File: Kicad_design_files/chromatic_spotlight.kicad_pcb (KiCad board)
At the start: 2 copper layers, 29.7 x 29.7 mm, 35 parts, among them CON1 POWER_CONN, P1 CONN_6, Q1 MOSFET_N, Q2 MOSFET_N, SW1 SLIDE 1PDT, U1 LT3474, U2 LT3474

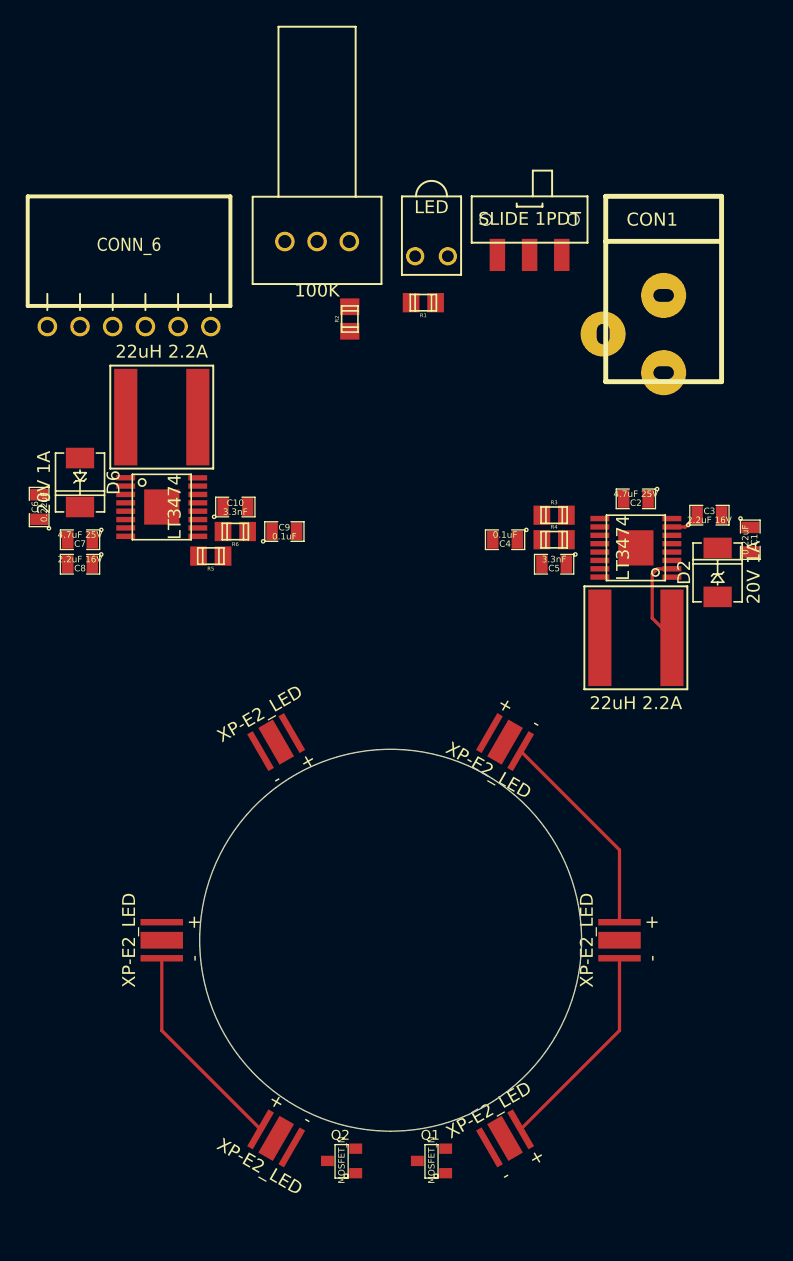
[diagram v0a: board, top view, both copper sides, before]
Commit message: almost done with layout
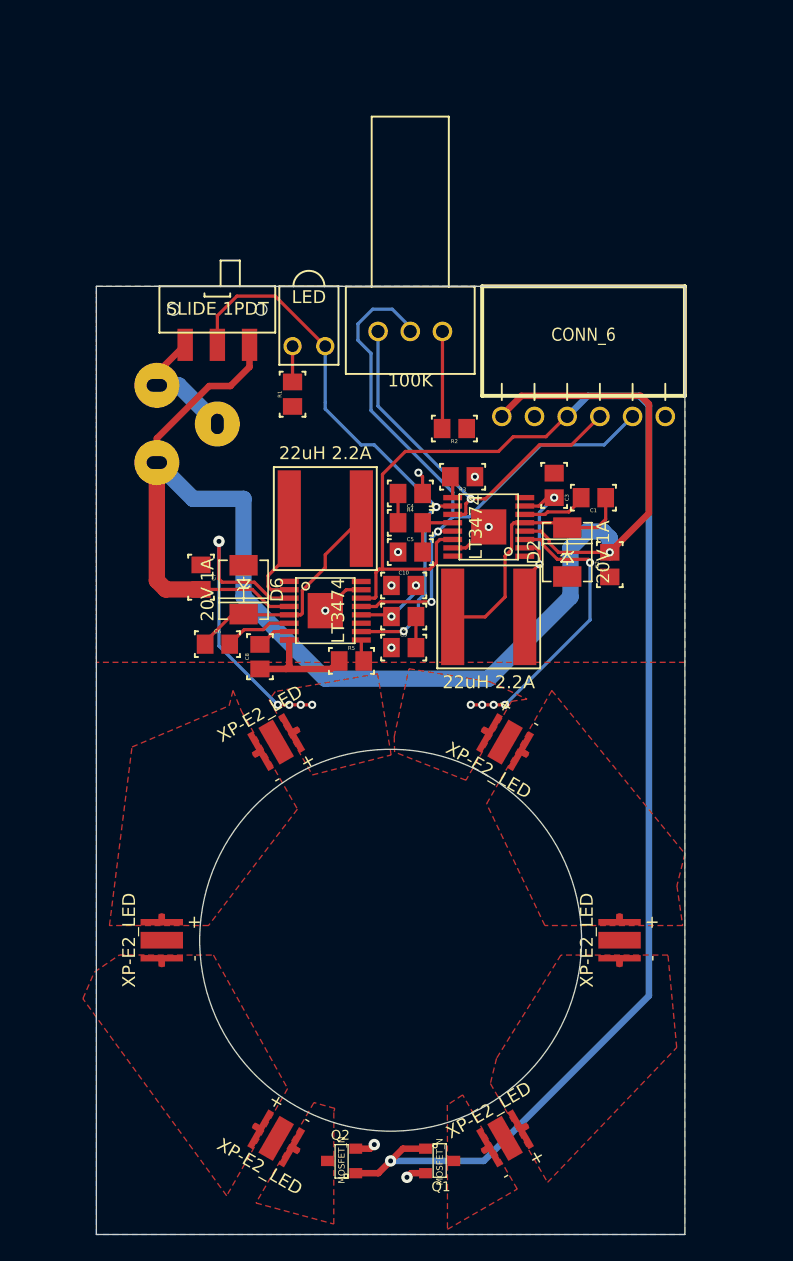
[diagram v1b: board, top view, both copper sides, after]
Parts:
- C1, C10, C2, C3, C4, C5, C6, C7, C8, C9: footprint SM0805 -> c_0805
- CON1: moved to B.Cu
- R1, R2, R3, R4, R5, R6: footprint c_0805 -> r_0805
- moved P1 36.0 mm to (15.0, -40.7)
- moved CON1 30.8 mm to (-13.5, -40.1), turned to 180 degrees
- moved SW1 25.2 mm to (-13.5, -46.3)
- moved C6 17.5 mm to (-13.5, -23.0), turned to 0 degrees
- moved C8 15.7 mm to (-10.2, -22.0), turned to 90 degrees
- moved D6 15.2 mm to (-11.4, -27.2)
- moved U2 15.0 mm to (-5.07, -25.6)
- moved L2 15.0 mm to (-5.07, -32.8)
- moved R6 14.7 mm to (1.02, -25.1)
- moved C10 14.4 mm to (1.02, -27.6)
- moved R5 13.6 mm to (-3.04, -21.7), turned to 0 degrees
- moved C9 12.9 mm to (1.02, -22.7)
- moved C1 12.6 mm to (15.8, -34.4), turned to 180 degrees
- moved R1 12.4 mm to (-7.62, -42.4), turned to 90 degrees
- moved C3 12.1 mm to (12.7, -34.4), turned to 270 degrees
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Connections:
- SW1 pad 1: GND -> +12V
- SW1 pad 3: +12V -> GND
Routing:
- net +12V: track 0.00 -> 120.9 mm, vias 0 -> 1
- net /LED_ARRAY_1/TRIGGER: track 0.00 -> 119.3 mm, vias 0 -> 1
- net /LED_ARRAY_1/V_ADJ: track 0.00 -> 54.7 mm, vias 0 -> 2
- net /LED_ARRAY_1/SHDN: track 0.00 -> 44.9 mm, vias 0 -> 2
- net GND: track 0.00 -> 31.9 mm, vias 0 -> 9
- net /LED_ARRAY_1/V_REF: track 0.00 -> 31.0 mm, vias 0 -> 1
- net N-0000028: track 0.00 -> 26.7 mm, vias 0 -> 5
- net N-0000013: track 0.00 -> 22.9 mm, vias 0 -> 5
- net N-0000016: track 0.00 -> 20.0 mm
- net N-0000029: track 0.00 -> 17.9 mm
- net N-0000031: track 16.5 -> 0.90 mm
- net N-0000018: track 16.5 -> 0.90 mm
- net N-0000017: track 16.5 -> 0.90 mm
- net N-0000036: track 0.00 -> 10.4 mm
- net N-0000012: track 0.00 -> 7.55 mm
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- added copper zone on F.Cu, net /LED_ARRAY_1/LED_CATHODE
- added copper zone on F.Cu, net /LED_ARRAY_2/LED_CATHODE
- added copper zone on B.Cu, net GND
- added copper zone on F.Cu, net GND
- added copper zone on F.Cu, net N-0000013
- added copper zone on F.Cu, net N-0000017
- added copper zone on F.Cu, net N-0000018
- added copper zone on F.Cu, net N-0000028
- added copper zone on F.Cu, net N-0000031
- added copper zone on F.Cu, net N-0000032
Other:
- board size 29.7 x 29.7 mm -> 45.7 x 73.7 mm
- net class Default: clearance 0.254 -> 0.1524; trace_width 0.254 -> 0.1524; via_dia 0.889 -> 0.635; via_drill 0.635 -> 0.381
- net class High_current_LED removed
- rule trace_clearance: 0.254 -> 0.1524
- rule trace_min: 0.254 -> 0.1524
- rule via_min_drill: 0.508 -> 0.381
- rule via_min_size: 0.889 -> 0.635
